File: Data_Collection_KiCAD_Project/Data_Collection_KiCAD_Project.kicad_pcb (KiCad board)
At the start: 2 copper layers, 68 parts, among them J1 USB_B_Micro, J2 Conn_Coaxial, J3 L717SDC37P1ACH4F, Q1 SI1040X-T1-GE3, U1 LM317T, U2 USBLC6-2SC6, U3 MCP9808_MSOP, U4 MAX-8Q, U5 STM32L552CC, U6 W25Q32JVSS, U7 MS5607-02BA, U8 BNO055, U9 KX134-1211, Y1 32MHz, Y2 32.768kHz

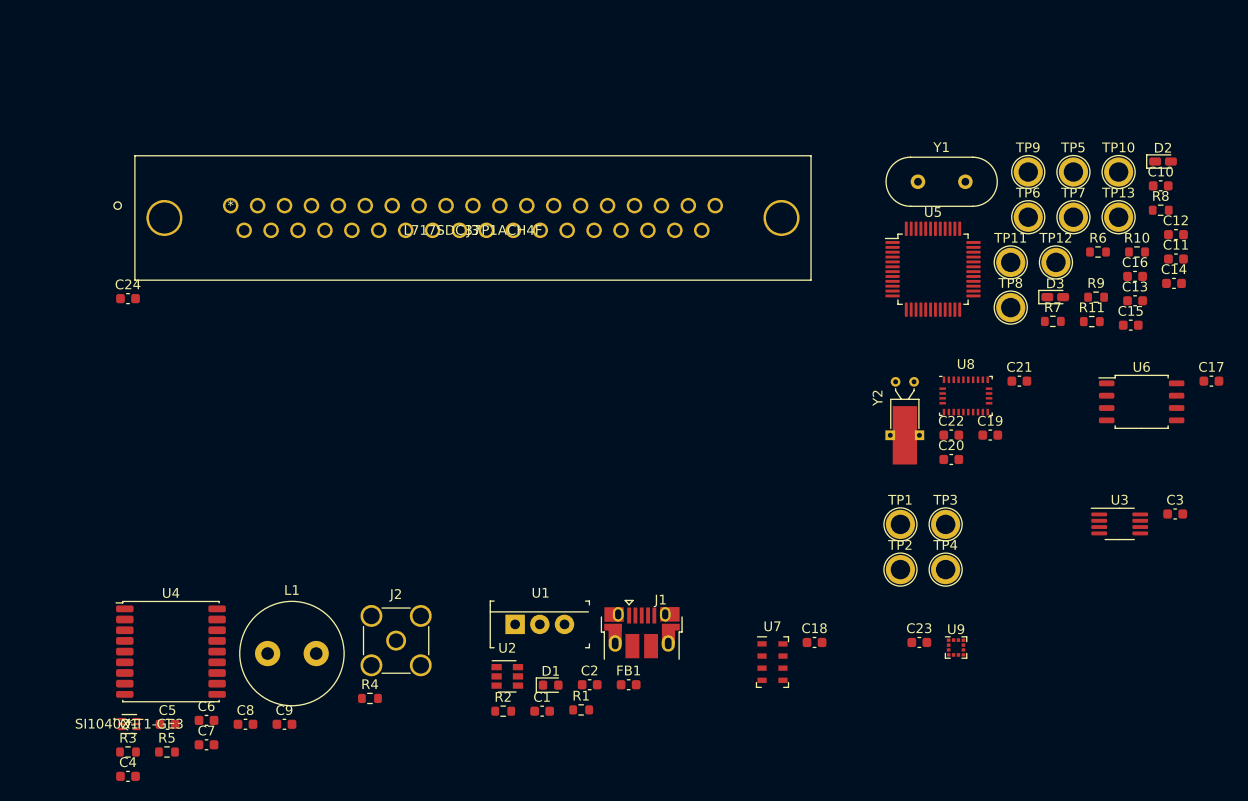
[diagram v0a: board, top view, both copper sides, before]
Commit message: Changed MCU and started pcb
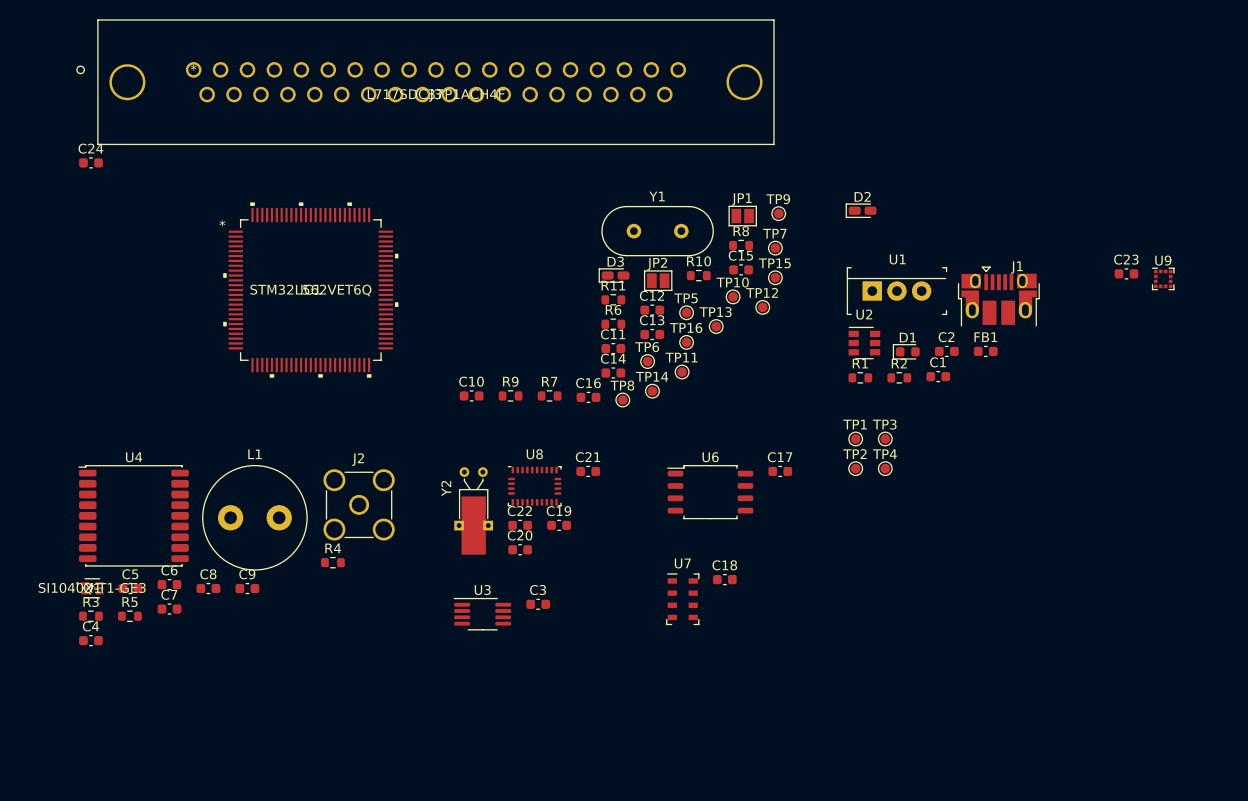
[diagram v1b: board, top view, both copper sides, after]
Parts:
- removed U5: STM32L552CC, Package_QFP:LQFP-48_7x7mm_P0.5mm
- added IC1: STM32L562VET6Q, STM32L562VET6Q:STM32L562VET6Q, F.Cu at (327.7, 43.2)
- added JP1: VDDA Bridge, Jumper:SolderJumper-2_P1.3mm_Open_Pad1.0x1.5mm, F.Cu at (372.1, 35.6)
- added JP2: VDD_SMPS, Jumper:SolderJumper-2_P1.3mm_Open_Pad1.0x1.5mm, F.Cu at (363.4, 42.2)
- added TP14: Debug Pad, TestPoint:TestPoint_Pad_D1.0mm, F.Cu at (362.8, 53.6)
- added TP15: Debug Pad, TestPoint:TestPoint_Pad_D1.0mm, F.Cu at (375.5, 41.9)
- added TP16: Debug Pad, TestPoint:TestPoint_Pad_D1.0mm, F.Cu at (366.3, 48.6)
- TP1, TP10, TP11, TP12, TP13, TP2, TP3, TP4, TP5, TP6, TP7, TP8, TP9: footprint TestPoint:TestPoint_Plated_Hole_D2.0mm -> TestPoint:TestPoint_Pad_D1.0mm
- moved C10 74.1 mm to (344.2, 54.1)
- moved C3 66.2 mm to (351.1, 75.5)
- moved U3 66.2 mm to (345.3, 76.5)
- moved R9 61.1 mm to (348.2, 54.1)
- moved C11 58.6 mm to (358.8, 49.2)
- moved C14 58.4 mm to (358.8, 51.7)
- moved C16 57.6 mm to (356.2, 54.2)
- moved C12 54.4 mm to (362.8, 45.2)
- moved C1 53.4 mm to (392.2, 52.1)
- moved R2 53.3 mm to (388.2, 52.2)
- moved R7 52.4 mm to (352.2, 54.1)
- moved R6 50.4 mm to (358.8, 46.7)
- moved D1 50.3 mm to (389.1, 49.5)
- moved U1 50.3 mm to (385.4, 43.3)
- moved C2 50.3 mm to (393.1, 49.5)
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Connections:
- J3 pad 22: /Main Bus/t_clk -> /SPI2_SCK
